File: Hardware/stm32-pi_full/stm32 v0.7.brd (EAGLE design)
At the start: 131.4 x 105.8 mm, 200 parts, among them Q1 MMBT3906, Q2 MMBT3904, Q3 MMBT3904, U1 ESP32-WROOM-32D

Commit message: commit JSON parser and arm_math examples
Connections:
- net GND: now also CFV1.2, CFV2.2, CFV3.2; no longer CFV1.1, CFV2.1, CFV3.1
- net VSIG1: now also CFV1.1; no longer CFV1.2
- net VSIG2: now also CFV2.1; no longer CFV2.2
- net VSIG3: now also CFV3.1; no longer CFV3.2

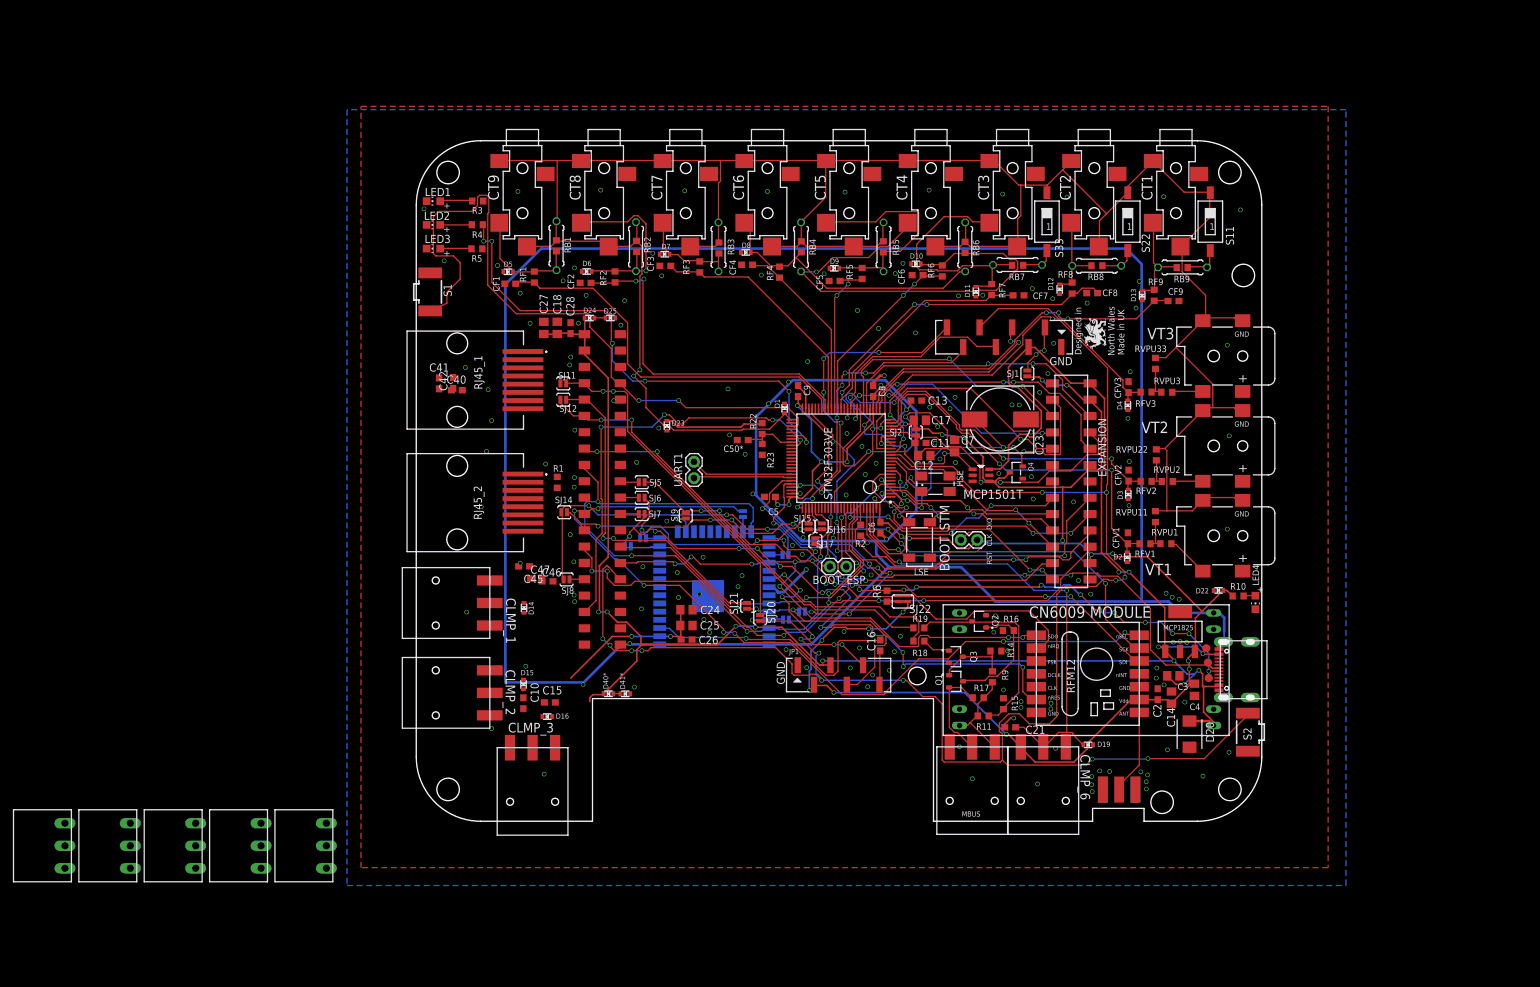
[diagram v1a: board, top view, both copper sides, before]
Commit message: update, plus reports
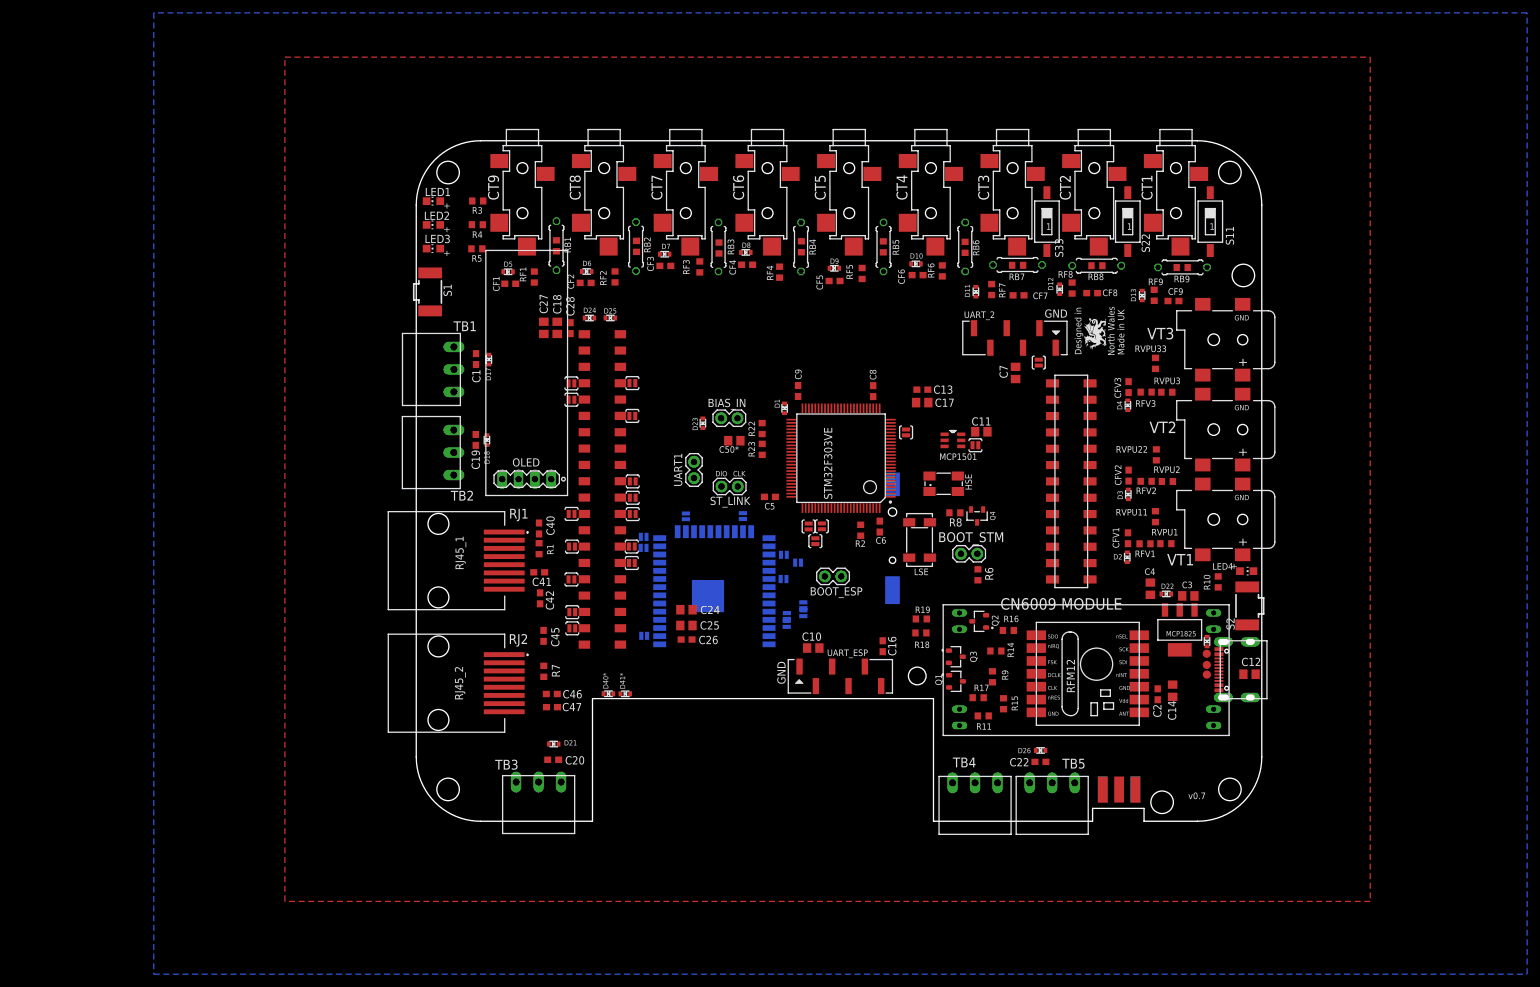
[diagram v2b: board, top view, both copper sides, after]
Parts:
- removed 3POLE_1, 3POLE_2, 3POLE_3, 3POLE_6, 3POLE_7: OMNIMATE_LSF_3COMBICON_SMT_3, OMNIMATE_LSF:OMNIMATE_LSF_3_SMT
- removed C15, C21: 100nF, resistor:C0603
- removed C23: (no value), rcl:153CLV-1010
- removed D14, D15, D16, D19: ESD5Z3.3T1G, microbuilder:SOD-523
- removed D20: (no value), diode:SMBJ
- removed JP1: (no value), pinhead+:1X06_SMT
- removed JP3: (no value), pinhead+:1X08_SMT
- added BIAS_IN, ST_LINK: (no value), SparkFun:1X02
- added C1, C19, C20, C22: 100nF, resistor:C0603
- added D17, D18, D21, D26, D40*1: ESD5Z3.3T1G, microbuilder:SOD-523
- added G1: CH291-1220LF, CH291-1220LF:CH291-1220LF
- added J1, SJ23, SJ24, SJ25, SJ26, SJ27, SJ28, SJ29, SJ30, SJ32: SOLDERJUMPERNO, SparkFun:SJ_2S-NO
- added OLED: (no value), con-lstb-db:MA04-1-OLED
- added R7: 4.7k, resistor:R0603
- added R8: 1k, resistor:R0603
- added UART_2, UART_ESP: (no value), pinhead+:1X06_SMT
- C10: value 100nF -> 2.2uF; device resistor:C0603 -> rcl:C0805
- C11: value 10nF -> 2.2uF; device rcl:C0603 -> rcl:C0805
- C12, C7: value 1uF -> 4.7uF
- C13: value 10nF -> 100nF
- C14, C17: value 1uF -> 2.2uF
- C24, C25, C3, C4: value 4.7uF -> 2.2uF
- C50*: value 1uF -> 2.2uF; device rcl:C0603 -> rcl:C0805
- SJ22: value (none) -> SOLDERJUMPERNO; device jumper-con_db:SJ-CON -> SparkFun:SJ_2S-NO
- moved U$5 143.6 mm to (98.9, 5.97), turned to 90 degrees
- moved U$6 141.8 mm to (86.9, 5.97), turned to 90 degrees
- moved U$1 76.7 mm to (5.86, 70.2)
- moved U$3 68.1 mm to (5.84, 57.3)
- moved C12 60.9 mm to (129.5, 22.9)
- moved U$4 54.2 mm to (19.0, 6.10), turned to 90 degrees
- moved C10 45.9 mm to (61.7, 26.9), turned to 180 degrees
- moved C42 36.1 mm to (19.2, 34.7), turned to 270 degrees
- moved C41 33.2 mm to (19.1, 38.7), turned to 0 degrees
- moved RJ45_1 28.2 mm to (4.70, 40.5)
- moved RJ45_2 28.2 mm to (4.70, 21.5)
- moved SJ22 26.8 mm to (86.9, 58.5)
- moved C40 25.0 mm to (19.1, 45.5), turned to 90 degrees
- moved C47 20.1 mm to (21.1, 17.7)
- moved S2 19.6 mm to (129.2, 33.5)
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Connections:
- net N$16 renamed CS_STM32_RPI
- removed net +3V3_ADC: C11.1, C12.1, C7.1, SJ2.2, STM32F303VE.21, VREF_3V3.1
- removed net N$11: JP1.4, SJ18.1, SJ21.2, U1.34
- removed net N$21: R6.1, SJ22.2
- removed net N$23: STM32F303VE.69, UART1.1
- removed net N$7: JP1.5, SJ20.2, SJ3.1, U1.35
- new net +3V3_ESP: SJ23.1, U1.2
- new net BOOT0_RPI: J1.2, PCB2.P$47
- new net N$16: Q4.2, R8.1
- new net NRST_STM_ESP: SJ25.1, U1.30
- new net NRST_STM_RPI: PCB2.P$51, SJ32.2
- new net RPI_GPIO16_RPI: PCB2.P$76, SJ29.1
- new net RPI_GPIO20_RPI: PCB2.P$78, SJ30.1
- new net RST_RFM_ESP: SJ24.1, U1.28
- new net RST_RFM_RPI: PCB2.P$69, SJ28.2
- new net RXD0_ESP: SJ18.1, SJ21.2, U1.34, UART_ESP.4
- new net SCL_RPI: PCB2.P$68, SJ27.1
- new net SDA_RPI: PCB2.P$67, SJ26.2
- new net TXD0_ESP: SJ20.2, SJ3.1, U1.35, UART_ESP.5
- new net VDD_MCP1501: C11.1, SJ22.2, VREF_3V3.4, VREF_3V3.6
- new net VREF+: SJ2.2, STM32F303VE.21, VREF_3V3.1
- net +3V3: now also BIAS_IN.1, OLED.3, R6.1, R7.2, SJ23.2, U$1.P$3, U$3.P$3, U$4.P$3, U$5.P$3; no longer 3POLE_1.P$1, 3POLE_2.P$1, 3POLE_3.P$1, 3POLE_6.P$1, JP1.2, R22.2, SJ22.1, U1.2, VREF_3V3.4
- net +5V: now also C10.1, C12.2, C7.1, D40*1.K, SJ22.1, UART_2.3, UART_ESP.3; no longer D20.C, JP1.3, JP3.3, VREF_3V3.6
- net 24V: now also U$6.P$3; no longer 3POLE_7.P$3
- net BOOT0: now also J1.1
- net BUTTON1: now also PCB2.P$53; no longer PCB2.P$47
- net DS18B20_2_RJ45: now also R7.1, STM32F303VE.81
- net GND: now also C1.2, C12.1, C19.2, C20.2, C22.2, D17.A, D18.A, D21.A, D26.A, D40*1.A, G1.-, OLED.4, U$1.P$1, U$3.P$1, U$4.P$1, U$5.P$1, U$6.P$1, UART_2.1, UART_ESP.1; no longer 3POLE_1.P$3, 3POLE_2.P$3, 3POLE_3.P$3, 3POLE_6.P$3, 3POLE_7.P$1, C12.2, C15.2, C21.2, C23.-, D14.A, D15.A, D16.A, D19.A, D20.A, JP1.1, JP3.1
- net MBUS_INPUT: now also U$6.P$2; no longer 3POLE_7.P$2
- net N$1: now also UART_2.2; no longer JP3.2
- net N$12: now also BIAS_IN.2, R22.2; no longer STM32F303VE.68, UART1.2
- net N$14: now also UART_ESP.6; no longer JP1.6
- net NRST_STM: now also SJ25.2, SJ32.1, UART_2.6; no longer JP3.6, PCB2.P$71, U1.30
- net PUSHIN_1: now also C1.1, D17.K, U$1.P$2; no longer 3POLE_1.P$2, D14.K
- net PUSHIN_2: now also C19.1, D18.K, U$3.P$2; no longer 3POLE_2.P$2, C10.1, D15.K
- net PUSHIN_3: now also C20.1, D21.K, U$4.P$2; no longer 3POLE_3.P$2, C15.1, D16.K
- net PUSHIN_BYANT: now also C22.1, D26.K, U$5.P$2; no longer 3POLE_6.P$2, C21.1, D19.K
- net RPI_GPIO16: now also SJ29.2; no longer PCB2.P$76
- net RPI_GPIO20: now also SJ30.2; no longer PCB2.P$78
- net RST_RFM: now also SJ24.2, SJ28.1; no longer PCB2.P$69, U1.28
- net SCL: now also OLED.2, SJ27.2; no longer PCB2.P$68
- net SDA: now also OLED.1, SJ26.1; no longer PCB2.P$67
- net SWCLK: now also ST_LINK.1; no longer JP3.7
- net SWDIO: now also ST_LINK.2; no longer JP3.8
- net UART1_RX: now also STM32F303VE.69, UART1.1
- net UART1_TX: now also STM32F303VE.68, UART1.2
- net UART2_RX: now also UART_2.4; no longer JP3.4
- net UART2_TX: now also UART_2.5; no longer JP3.5
- net VBAT: now also G1.+, R8.2; no longer C23.+, Q4.2
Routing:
- net GND: track 460.9 -> 0.00 mm, vias 169 -> 0
- net BIAS: track 390.1 -> 0.00 mm, vias 2 -> 0
- net +3V3: track 349.9 -> 0.00 mm, vias 27 -> 0
- net NRST_STM: track 304.1 -> 0.00 mm, vias 18 -> 0
- net +5V: track 294.8 -> 0.00 mm, vias 12 -> 0
- net DIO0: track 145.6 -> 0.00 mm, vias 6 -> 0
- net CS_RFM69: track 132.1 -> 0.00 mm, vias 7 -> 0
- net SCL: track 111.7 -> 0.00 mm, vias 7 -> 0
- net BUTTON1: track 107.8 -> 0.00 mm, vias 2 -> 0
- net SPI_CLK: track 100.3 -> 0.00 mm, vias 8 -> 0
- net SDA: track 93.9 -> 0.00 mm, vias 4 -> 0
- net MISO: track 93.3 -> 0.00 mm, vias 9 -> 0
- net MOSI: track 93.1 -> 0.00 mm, vias 8 -> 0
- net D-: track 93.1 -> 0.00 mm, vias 4 -> 0
- net D+: track 92.6 -> 0.00 mm, vias 12 -> 0
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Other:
- board text added: "CH291-1220LF"
- board text added: "MCP1501"
- board text added: "RJ1"
- board text added: "RJ2"
- board text added: "TB1"
- board text added: "TB2"
- board text added: "TB3"
- board text added: "TB4"
- board text added: "TB5"
- board text added: "UART_ESP"
- board text added: "v0.7"
- board text removed: "CLMP_1"
- board text removed: "CLMP_2"
- board text removed: "CLMP_3"
- board text removed: "CLMP_6"
- board text removed: "MBUS"
- board text removed: "MCP1501T"
- board text removed: "RST"
- board text removed: "v0.6"

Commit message: board v0.7
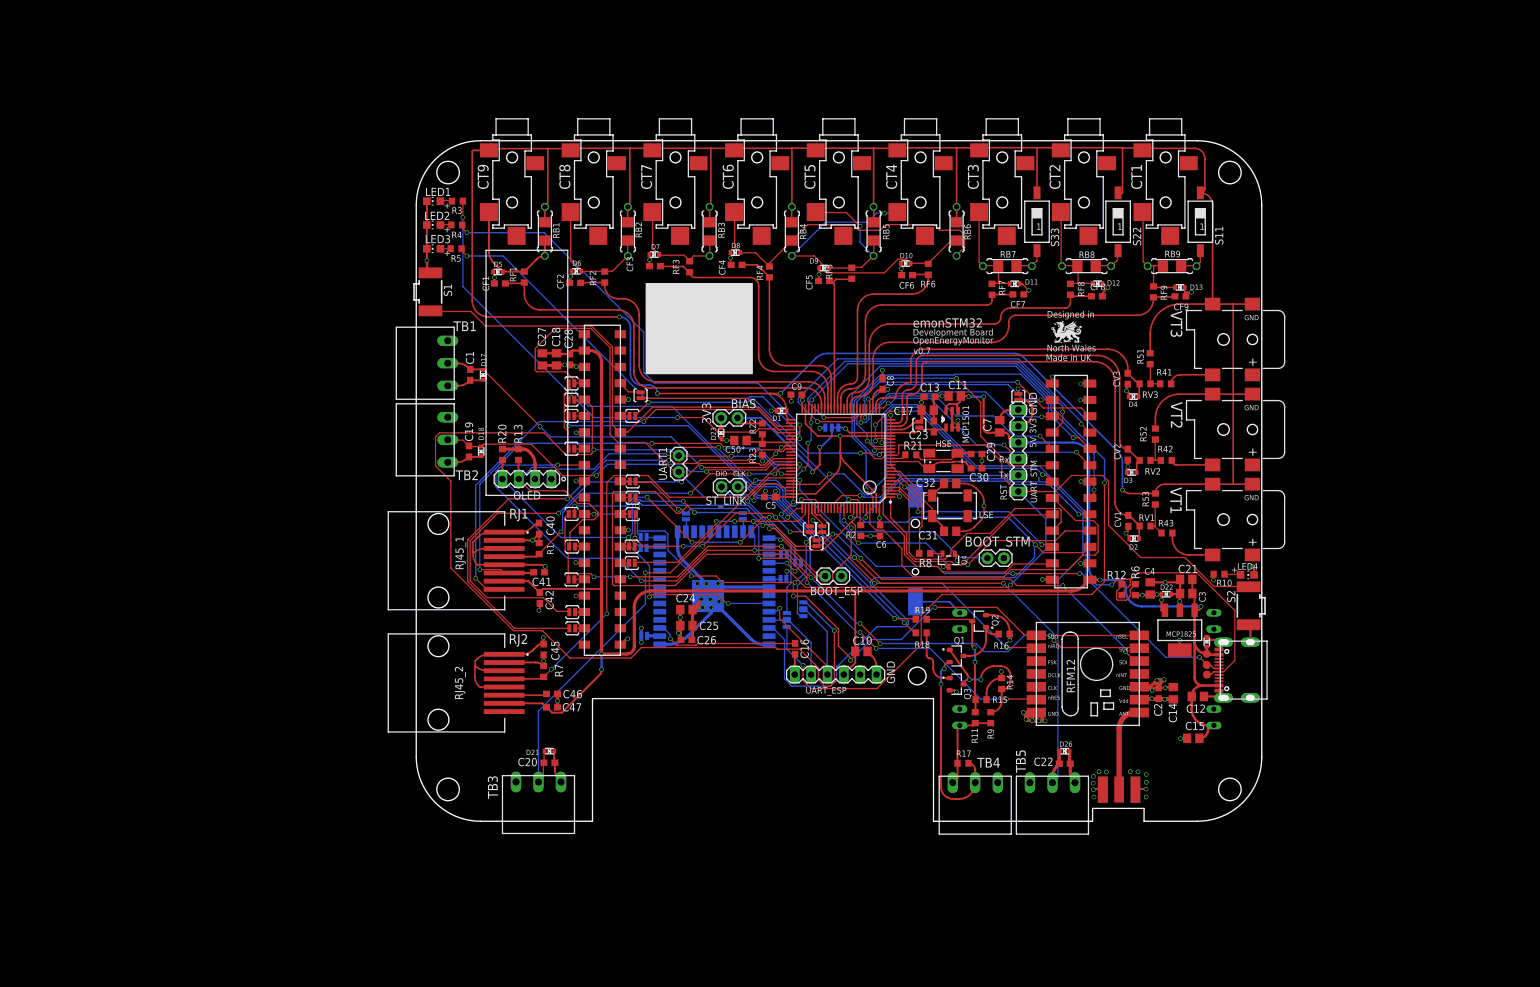
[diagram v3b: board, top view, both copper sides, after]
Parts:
- removed CFV1, CFV2, CFV3: 100nF, resistor:C0603
- removed D24, D25, D40*, D41*: ESD5Z3.3T1G, microbuilder:SOD-523
- removed RFV1, RFV2, RFV3: 330R, resistor:R0603
- removed RVPU1, RVPU2, RVPU3: 120k, resistor:R0603
- removed RVPU11, RVPU22, RVPU33: 10k, resistor:R0603
- removed SJ22: SOLDERJUMPERNO, SparkFun:SJ_2S-NO
- removed UART_2, UART_ESP: (no value), pinhead+:1X06_SMT
- added C15, C21, C31, C32: 2.2uF, rcl:C0805
- added C23: 200pF*, rcl:C0603
- added C29, C30: 5nF, rcl:C0603
- added CV1, CV2, CV3: 100nF, resistor:C0603
- added JP1: JUMPER-SMT_3_1-NC_TRACE_NO-SILK, SparkFun-Jumpers:SMT-JUMPER_3_1-NC_TRACE_NO-SILK
- added R12: 330R, rcl:R0603
- added R13, R20, R51, R52, R53: 10k, resistor:R0603
- added R21: 200k, resistor:R0603
- added R41, R42, R43: 120k, resistor:R0603
- added RV1, RV2, RV3: 330R, resistor:R0603
- added SJ31, SJ33: SOLDERJUMPERNO, SparkFun:SJ_2S-NO
- added SV1, SV2: (no value), con-lstb-db:MA06-1
- C12, C18, C27, C7: value 4.7uF -> 2.2uF
- CT1, CT2, CT3, CT4, CT5, CT6, CT7, CT8, CT9: value STEREO_SMD -> SJ-3523-SMT
- D40*1: value ESD5Z3.3T1G -> ESD5Z5.0T1G
- HSE: value 8MHZ ~15pFmax -> 406C35E08M00000
- PCB2: value RPI3YA -> TSM-120-01-T-DV
- R10, R3, R4, R5: value 220R -> 330R
- R18, R19: value 1K -> 1k
- R6: value 1.5K -> 1k
- R8: value 1k -> 1.5k
- RB1, RB2, RB3, RB4, RB5, RB6, RB7, RB8, RB9: device resistor:R0603 -> rcl:R1206
- STM32F303VE: value STM32F303XB -> STM32F303VE
- VT1, VT2, VT3: value 2.1MMJACKSMT -> ADC-028-2-T
- moved R6 24.6 mm to (111.8, 36.0), turned to 90 degrees
- moved C16 13.6 mm to (58.9, 26.8)
- moved R17 10.5 mm to (85.0, 9.00), turned to 180 degrees
- moved C12 8.75 mm to (121.5, 19.4), turned to 180 degrees
- moved C7 8.66 mm to (90.7, 61.4), turned to 90 degrees
- moved Q4 8.18 mm to (82.8, 40.6)
- moved R8 7.86 mm to (79.0, 41.6)
- moved C10 7.50 mm to (69.2, 26.4), turned to 0 degrees
- moved LSE 7.11 mm to (83.0, 49.0), turned to 0 degrees
- moved C11 6.93 mm to (83.7, 66.1), turned to 180 degrees
- moved R9 6.36 mm to (89.3, 16.1)
- moved SJ1 6.19 mm to (93.6, 66.0), turned to 90 degrees
- moved D11 6.16 mm to (93.0, 83.6), turned to 90 degrees
- moved D13 5.99 mm to (118.7, 83.0), turned to 90 degrees
- moved D12 5.95 mm to (105.9, 83.6), turned to 90 degrees
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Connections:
- net MBUS_INPUT renamed MBUS_I/O
- net N$20 renamed ANT
- removed net N$18: D24.A, D25.K
- removed net N$19: D40*.A, D41*.K
- removed net VDD_MCP1501: C11.1, SJ22.2, VREF_3V3.4, VREF_3V3.6
- removed net VT1_EX: EXPANSION.11
- removed net VT2_EX: EXPANSION.12
- removed net VT3_EX: EXPANSION.13
- new net HSE_OUT_: C29.1, HSE.3, R21.2
- new net MBUS_RX_RPI: PCB2.P$56, SJ33.1
- new net MBUS_TX_RPI: PCB2.P$52, SJ31.1
- new net N$7: R12.1, R6.2
- net +3V3: now also JP1.1, R13.1, R20.1, U$1.P$1, U$3.P$1, U$4.P$1, U$5.P$1; no longer U$1.P$3, U$3.P$3, U$4.P$3, U$5.P$3
- net +5V: now also C11.1, C15.2, C21.1, C3.1, EXPANSION.26, SV1.3, SV2.3, VREF_3V3.4, VREF_3V3.6; no longer C3.2, D24.K, D40*.K, EXPANSION.2, SJ22.1, UART_2.3, UART_ESP.3
- net 24V: now also U$6.P$1; no longer U$6.P$3
- net AC1: now also R43.2; no longer RVPU1.2
- net AC2: now also R42.2; no longer RVPU2.2
- net AC3: now also R41.1; no longer RVPU3.1
- net ADC0: now also R41.2, R51.1, RV3.1; no longer RFV3.1, RVPU3.2, RVPU33.1
- net BIAS: now also R51.2, R52.2, R53.2; no longer CT1.P$4, CT2.P$4, CT3.P$4, CT4.P$4, CT5.P$4, CT6.P$4, CT7.P$4, CT8.P$4, CT9.P$4, RVPU11.2, RVPU22.2, RVPU33.2
- net D+: now also R12.2; no longer R6.2
- net GND: now also C15.1, C21.2, C23.2, C29.2, C3.2, C30.2, C31.2, C32.2, CV1.2, CV2.2, CV3.2, EXPANSION.2, EXPANSION.25, SV1.1, SV2.1, U$1.P$3, U$3.P$3, U$4.P$3, U$5.P$3, U$6.P$3; no longer C3.1, CFV1.2, CFV2.2, CFV3.2, D25.A, D41*.A, EXPANSION.26, U$1.P$1, U$3.P$1, U$4.P$1, U$5.P$1, U$6.P$1, UART_2.1, UART_ESP.1
- net HSE_IN: now also C30.1
- net HSE_OUT: now also R21.1; no longer HSE.3
- net IO8_EX: no longer EXPANSION.25
- net MBUS_RX: now also SJ33.2; no longer PCB2.P$56
- net MBUS_TX: now also SJ31.2; no longer PCB2.P$52
- net N$1: now also SV1.2; no longer UART_2.2
- net N$12: now also JP1.2
- net N$14: now also SV2.6; no longer UART_ESP.6
- net N$34: now also R42.1, R52.1, RV2.1; no longer RFV2.1, RVPU2.1, RVPU22.1
- net N$37: now also R43.1, R53.1, RV1.1; no longer RFV1.1, RVPU1.1, RVPU11.1
- net NRST_STM: now also SV1.6; no longer UART_2.6
- net PC14: now also C31.1
- net PC15: now also C32.1
- net RXD0_ESP: now also SV2.4; no longer UART_ESP.4
- net SCL: now also R13.2
- net SDA: now also R20.2
- net TXD0_ESP: now also SV2.5; no longer UART_ESP.5
- net UART2_RX: now also SV1.4; no longer UART_2.4
- net UART2_TX: now also SV1.5; no longer UART_2.5
- net VREF+: now also C23.1, JP1.3
- net VSIG1: now also CV1.1, RV1.2; no longer CFV1.1, RFV1.2
- net VSIG2: now also CV2.1, RV2.2; no longer CFV2.1, RFV2.2
- net VSIG3: now also CV3.1, RV3.2; no longer CFV3.1, RFV3.2
- net VSIG4: now also EXPANSION.11
- net VSIG5: now also EXPANSION.12
- net VSIG6: now also EXPANSION.13
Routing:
- net BIAS: track 0.00 -> 467.4 mm, vias 0 -> 4
- net GND: track 0.00 -> 367.0 mm, vias 0 -> 80
- net +5V: track 0.00 -> 302.1 mm, vias 0 -> 6
- net SCL: track 0.00 -> 207.0 mm, vias 0 -> 4
- net UART1_TX: track 0.00 -> 175.0 mm, vias 0 -> 4
- net NRST_STM: track 0.00 -> 174.1 mm, vias 0 -> 4
- net SDA: track 0.00 -> 148.6 mm, vias 0 -> 6
- net CS_RFM69: track 0.00 -> 145.6 mm, vias 0 -> 7
- net USART3_RX: track 0.00 -> 141.6 mm, vias 0 -> 3
- net DIO0: track 0.00 -> 130.5 mm, vias 0 -> 7
- net D+: track 0.00 -> 118.7 mm, vias 0 -> 2
- net SPI_CLK: track 0.00 -> 99.1 mm, vias 0 -> 9
- net MISO: track 0.00 -> 97.3 mm, vias 0 -> 7
- net UART1_RX: track 0.00 -> 94.5 mm, vias 0 -> 1
- net MOSI: track 0.00 -> 92.6 mm, vias 0 -> 6
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- added copper zone on layer 15, net +3V3
- added copper zone on layer 2, net GND
- removed copper zone on layer 1, net GND
- removed copper zone on layer 16, net GND
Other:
- board text added: "3V3"
- board text added: "5V"
- board text added: "BIAS"
- board text added: "RST"
- board text added: "Rx"
- board text added: "Tx"
- board text added: "UART_STM"
- board text removed: "CN6009 MODULE"
